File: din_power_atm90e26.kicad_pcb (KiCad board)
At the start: 2 copper layers, 86.9 x 32.8 mm, 60 parts, among them J1 CONN_01X06, J2 VBAT, J3 CONN_01X08, J4 CONN_02X18, J5 CONN_01X08, U1 MCP73831-2-OT, U2 TLV1117-33, U3 TLV1117-33, U4 Hi-Link_SMPS, U5 dc-dc

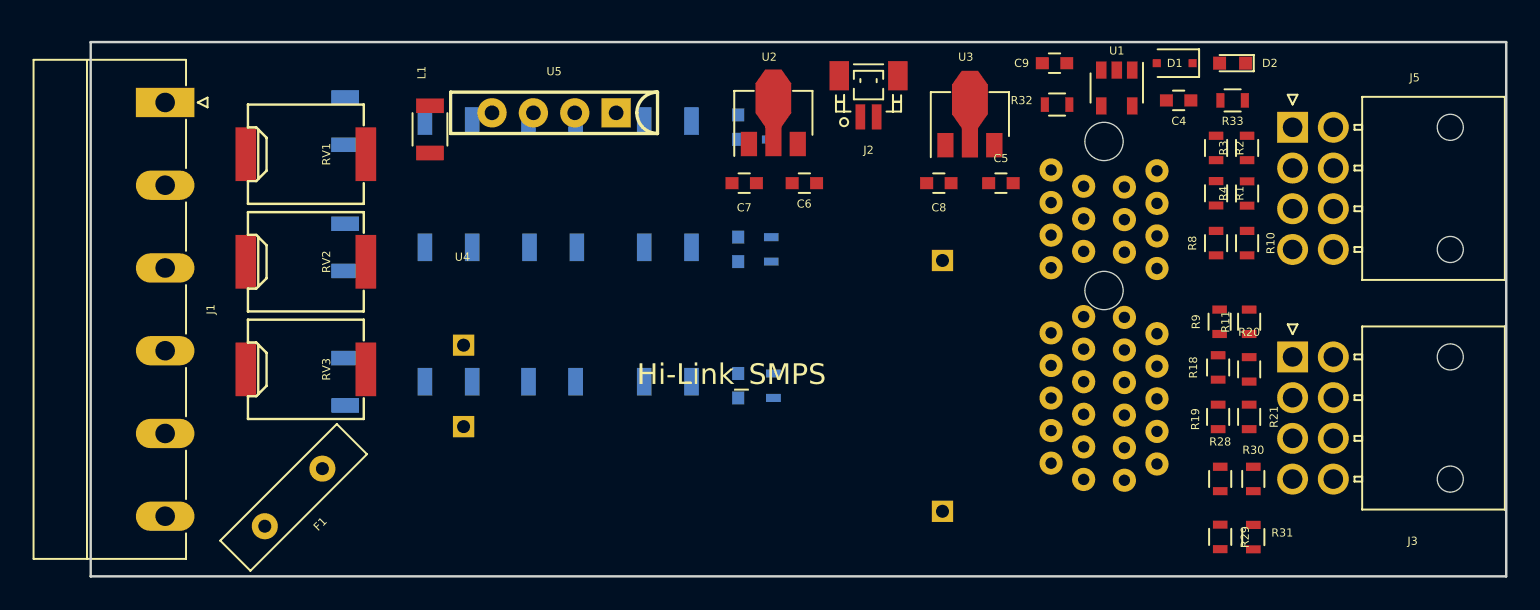
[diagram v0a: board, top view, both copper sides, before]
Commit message: Changes from urbito
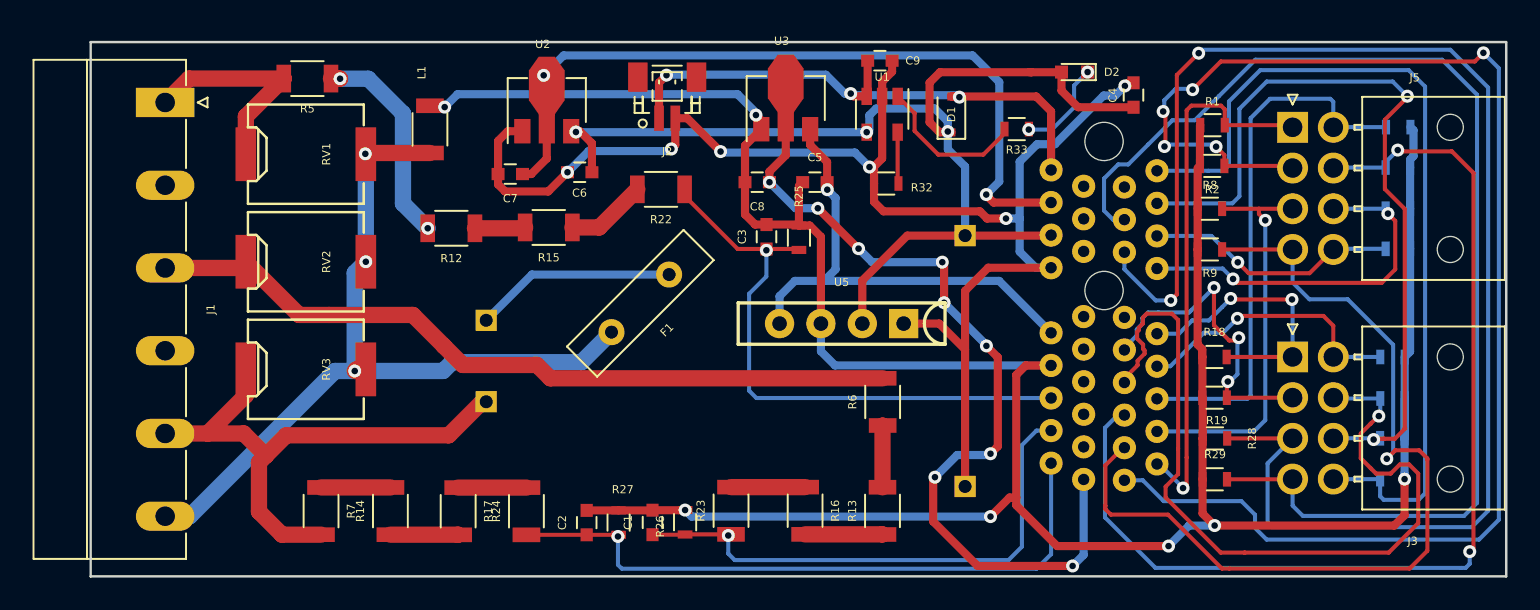
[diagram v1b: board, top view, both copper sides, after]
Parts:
- C1, C2, C3, R12, R13, R14, R15, R16, R17, R22, R23, R24, R25, R26, R27, R5, R6, R7: moved to F.Cu
- R10, R11, R20, R21, R3, R30, R31, R4, U4: moved to B.Cu
- moved R6 34.3 mm to (154.5, 67.6), turned to 90 degrees
- moved R13 31.2 mm to (154.5, 74.2), turned to 90 degrees
- moved F1 24.4 mm to (141.4, 59.7)
- moved R16 22.4 mm to (149.8, 74.2), turned to 270 degrees
- moved U5 21.9 mm to (152.0, 62.7)
- moved R26 17.6 mm to (142.4, 74.9), turned to 270 degrees
- moved C1 17.6 mm to (140.4, 75.0), turned to 90 degrees
- moved R23 16.6 mm to (145.2, 74.2), turned to 90 degrees
- moved U1 14.5 mm to (154.5, 49.9)
- moved C7 14.4 mm to (131.7, 53.6)
- moved D1 14.1 mm to (158.8, 49.9), turned to 90 degrees
- moved U2 13.9 mm to (133.9, 49.5)
- moved C6 13.8 mm to (135.9, 53.5)
- moved R33 13.4 mm to (162.8, 50.8)
- moved R27 12.7 mm to (138.3, 75.0), turned to 270 degrees
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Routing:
- net GNDA: track 0.00 -> 171.9 mm, vias 0 -> 7
- net GNDPWR: track 0.00 -> 89.6 mm, vias 0 -> 6
- net IB2+: track 0.00 -> 89.3 mm, vias 0 -> 2
- net IA1-: track 0.00 -> 87.3 mm, vias 0 -> 5
- net IB2-: track 0.00 -> 72.9 mm
- net +5V: track 0.00 -> 69.5 mm, vias 0 -> 3
- net IC1-: track 0.00 -> 64.7 mm, vias 0 -> 2
- net +3.3V_ISO: track 0.00 -> 57.1 mm, vias 0 -> 9
- net IB1-: track 0.00 -> 55.9 mm, vias 0 -> 1
- net IN2-: track 0.00 -> 53.6 mm
- net IC2-: track 0.00 -> 50.7 mm, vias 0 -> 1
- net UN: track 0.00 -> 50.4 mm, vias 0 -> 3
- net +3V3: track 0.00 -> 50.3 mm, vias 0 -> 2
- net IN2+: track 0.00 -> 49.5 mm, vias 0 -> 2
- net UB: track 0.00 -> 47.2 mm
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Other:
- rule trace_min: 0.2 -> 0.1
- rule via_min_drill: 0.3 -> 0.2
- rule via_min_size: 0.4 -> 0.3
